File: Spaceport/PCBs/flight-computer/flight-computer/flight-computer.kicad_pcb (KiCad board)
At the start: 4 copper layers, 70.1 x 49.9 mm, 107 parts, among them IC1 AP7362-33SP-13, IC2 AP7362-33SP-13, J10 5.0VOUT, J11 SWD, J12 Charge, J13 Conn_01x02, J14 Micro_SD_Card, J2 Conn_01x02, J3 Conn_01x02, J4 USB_C_Receptacle_USB2.0_16P, J5 UART, J6 UART, J7 I2C, J8 SPI, J9 3.3VOUT, U1 MS5611-01BA, U2 BMI088, U3 H3LIS331DL, U4 MMC5603NJ, U5 SAM-M10Q-00B, U6 TPS62A03DRLR, U7 STM32H723VEHx, U8 BQ25606RGER, U9 ESP32-S3-MINI-1-N4R2, Y1 ECS-2520S

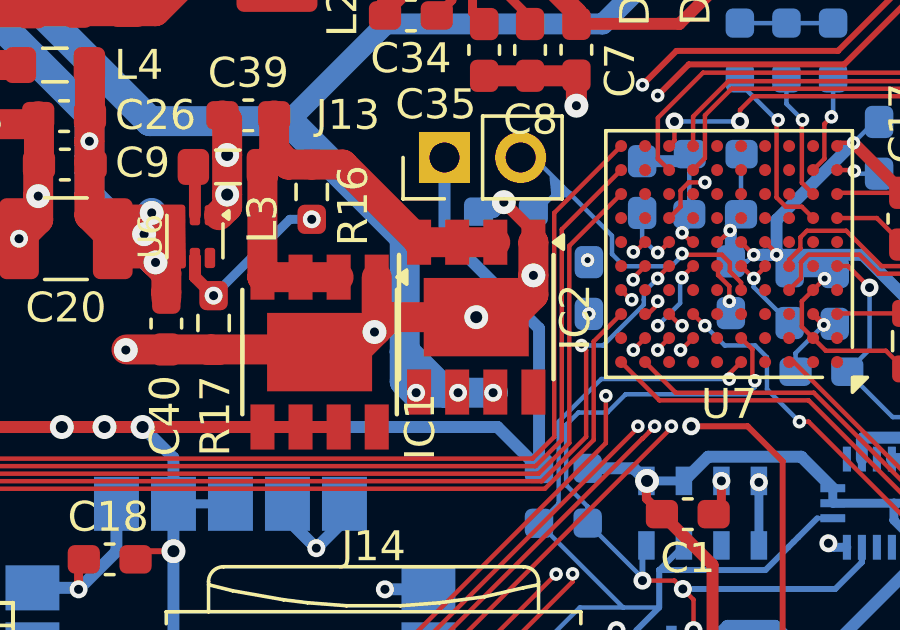
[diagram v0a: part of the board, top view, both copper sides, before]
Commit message: more changes
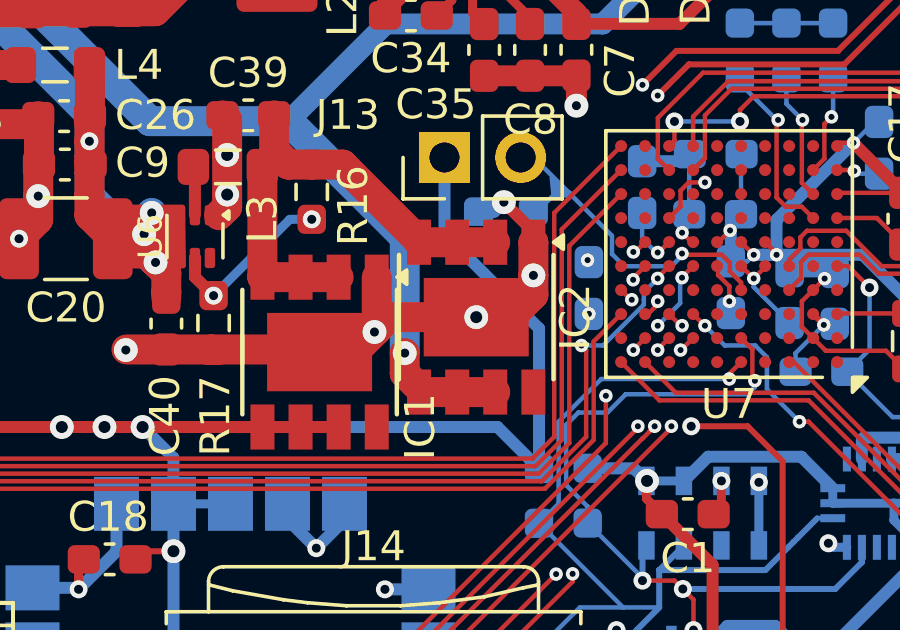
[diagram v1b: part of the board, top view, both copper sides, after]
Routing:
- net +3V3B: track 103.0 -> 100.6 mm, vias 3 -> 1
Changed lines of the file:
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@@
 		(net 31)
 	)
-	(via
-		(at 156.0068 76.4032)
-		(size 0.6)
-		(drill 0.3)
-		(layers "F.Cu" "B.Cu")
+	(segment
+		(start 153.6828 76.3817)
+		(end 156.0798 76.3817)
+		(width 1)
+		(layer "F.Cu")
+		(net 33)
+	)
+	(segment
+		(start 153.0604 75.7593)
+		(end 153.6828 76.3817)
+		(width 1)
+		(layer "F.Cu")
+		(net 33)
+	)
+	(segment
+		(start 153.0604 75.0824)
+		(end 153.0604 75.7593)
+		(width 1)
+		(layer "F.Cu")
 		(net 33)
 	)
 	(via
-		(at 154.8384 76.4032)
-		(size 0.6)
+		(at 153.0604 75.0824)
+		(size 0.8)
 		(drill 0.3)
 		(layers "F.Cu" "B.Cu")
-		(net 33)
-	)
-	(via
-		(at 153.4414 76.4032)
-		(size 0.6)
-		(drill 0.3)
-		(layers "F.Cu" "B.Cu")
-		(net 33)
-	)
-	(segment
-		(start 153.0604 76.0222)
-		(end 153.4414 76.4032)
-		(width 1)
-		(layer "B.Cu")
-		(net 33)
-	)
-	(segment
-		(start 153.0604 75.0316)
-		(end 154.432 76.4032)
-		(width 1)
-		(layer "B.Cu")
 		(net 33)
 	)
@@
 	)
 	(segment
-		(start 154.432 76.4032)
-		(end 154.8384 76.4032)
+		(start 153.0604 71.2216)
+		(end 153.0604 75.0824)
 		(width 1)
 		(layer "B.Cu")
@@
 		(start 129.2 58.6)
 		(end 135.816 58.6)
-		(width 1)
-		(layer "B.Cu")
-		(net 33)
-	)
-	(segment
-		(start 153.4414 76.4032)
-		(end 156.0068 76.4032)
 		(width 1)
 		(layer "B.Cu")
@@
 	)
 	(segment
-		(start 153.0604 75.0316)
-		(end 153.0604 76.0222)
-		(width 1)
-		(layer "B.Cu")
-		(net 33)
-	)
-	(segment
 		(start 123.613 53.013)
 		(end 129.2 58.6)
@@
 		(layer "B.Cu")
 		(net 33)
-	)
-	(segment
-		(start 153.0604 71.2216)
-		(end 153.0604 75.0316)
-		(width 1)
-		(layer "B.Cu")
-		(net 33)
